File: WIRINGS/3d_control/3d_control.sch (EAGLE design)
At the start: 8 parts

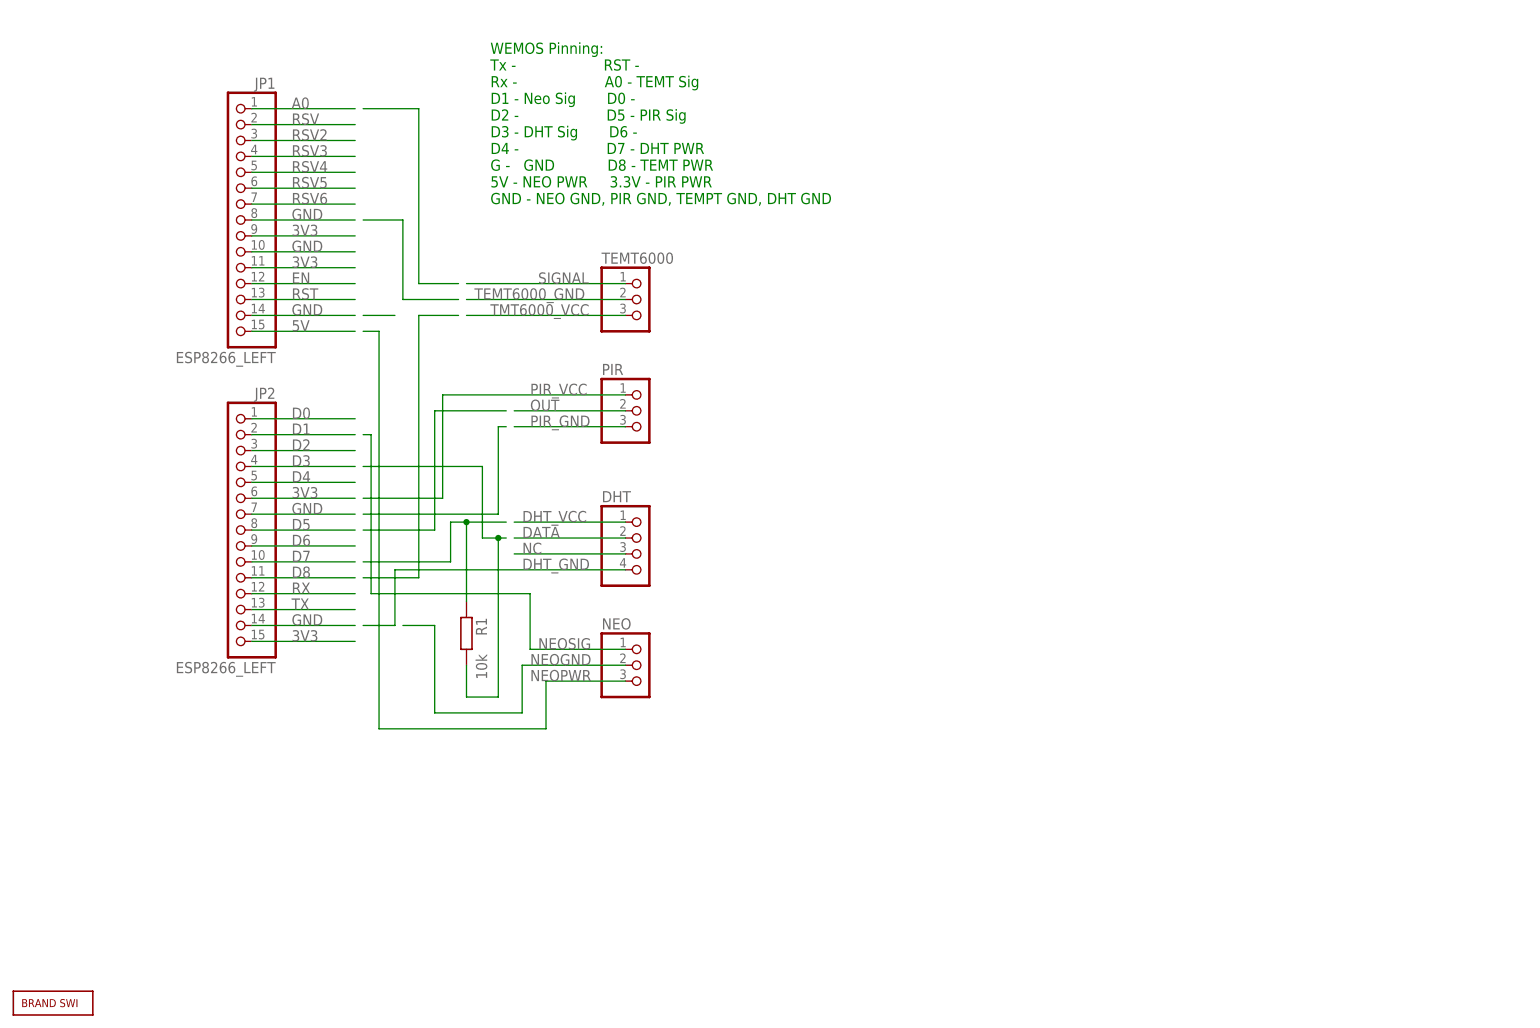
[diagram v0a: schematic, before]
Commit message: integration checkin
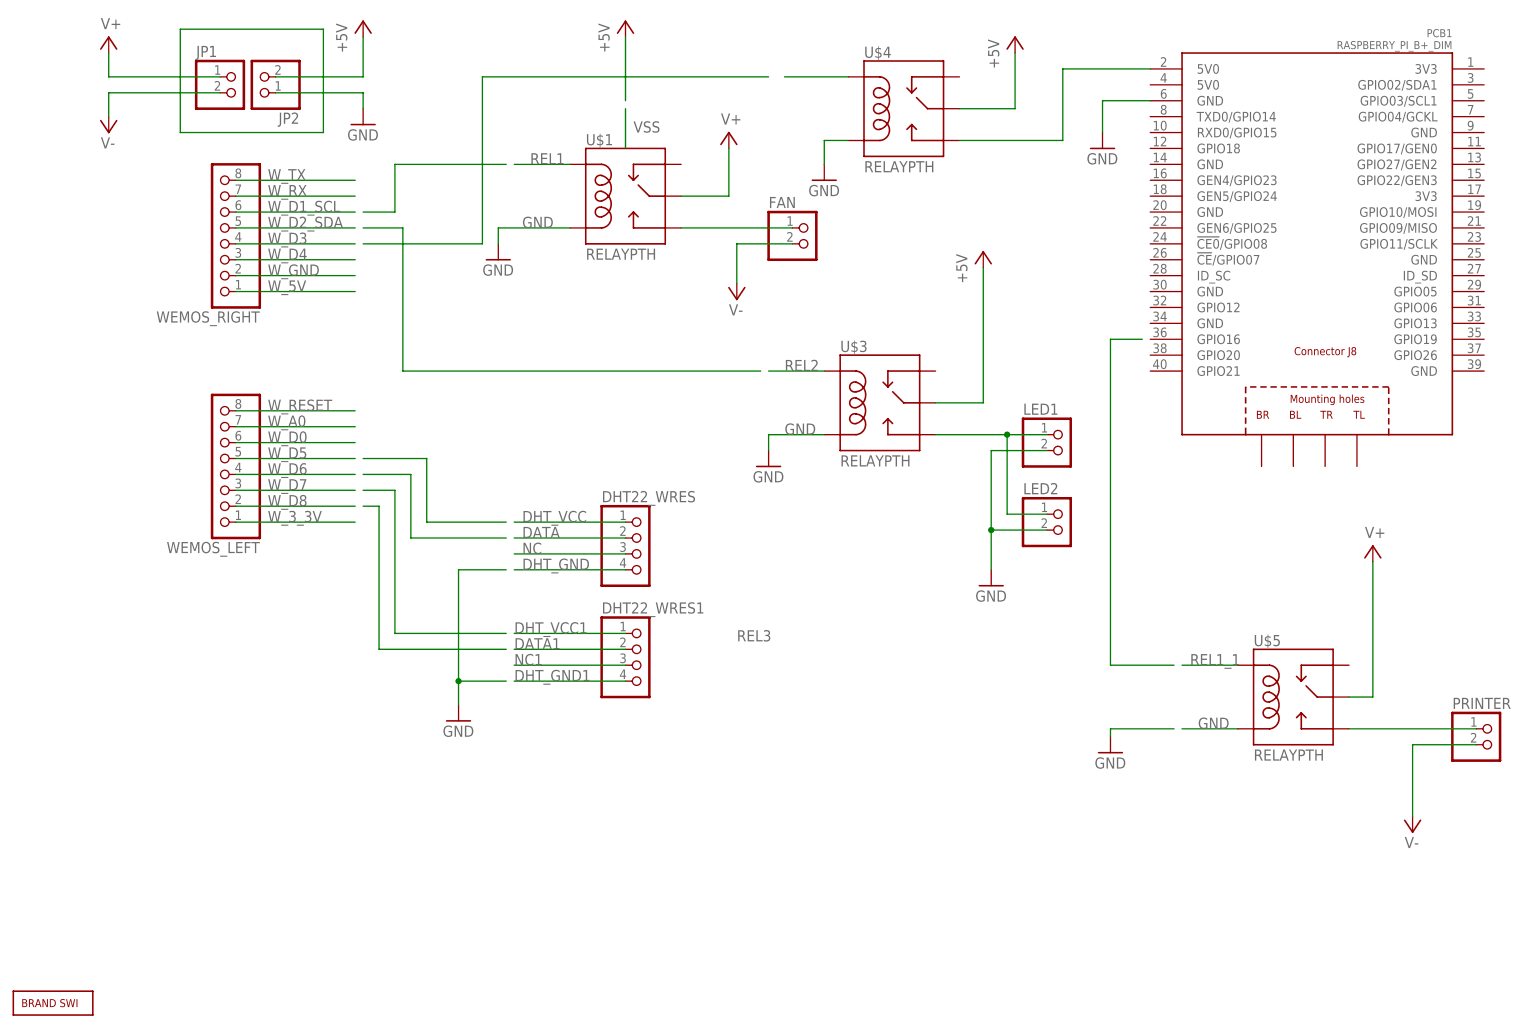
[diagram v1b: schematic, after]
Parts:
- removed NEO, PIR, TEMT6000: (no value), pinhead:PINHD-1X3
- removed R1: 10k, rcl:R-EU_0207/10
- added DHT22_WRES1: (no value), pinhead:PINHD-1X4
- added FAN, LED1, LED2, PRINTER: (no value), pinhead:PINHD-1X2
- added PCB1: RASPBERRY_PI_B+_DIM, SWI_COMMONS:RASPBERRY_PI_B+_DIM
- added U$1, U$3, U$4, U$5: RELAYPTH, SWI_COMMONS:RELAYPTH
- added WEMOS_LEFT, WEMOS_RIGHT: (no value), pinhead:PINHD-1X8
- JP1, JP2: value ESP8266_LEFT -> (none); device pinhead:PINHD-1X15 -> pinhead:PINHD-1X2
- renumbered DHT to DHT22_WRES
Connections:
- removed net 3V3: JP1.11, JP1.9, JP2.15, JP2.6
- removed net 5V: JP1.15
- removed net A0: JP1.1
- removed net D0: JP2.1
- removed net D1: JP2.2
- removed net D2: JP2.3
- removed net D3: JP2.4
- removed net D4: JP2.5
- removed net D5: JP2.8
- removed net D6: JP2.9
- removed net D7: JP2.10
- removed net D8: JP2.11
- removed net EN: JP1.12
- removed net N$3: R1.1
- removed net NEOGND: NEO.2
- removed net NEOPWR: NEO.3
- removed net NEOSIG: NEO.1
- removed net OUT: PIR.2
- removed net PIR_GND: PIR.3
- removed net PIR_VCC: PIR.1
- removed net RST: JP1.13
- removed net RSV: JP1.2
- removed net RSV2: JP1.3
- removed net RSV3: JP1.4
- removed net RSV4: JP1.5
- removed net RSV5: JP1.6
- removed net RSV6: JP1.7
- removed net RX: JP2.12
- removed net SIGNAL: TEMT6000.1
- removed net TEMT6000_GND: TEMT6000.2
- removed net TMT6000_VCC: TEMT6000.3
- removed net TX: JP2.13
- new net +5V: JP2.2, U$3.SWCOMMON, U$4.SWCOMMON
- new net DATA1: DHT22_WRES1.2
- new net DHT_GND1: DHT22_WRES1.4
- new net DHT_VCC1: DHT22_WRES1.1
- new net N$10: PCB1.5V0@1, U$4.SWOPEN
- new net N$13: PRINTER.1, U$5.SWOPEN
- new net N$9: FAN.1, U$1.SWOPEN
- new net NC1: DHT22_WRES1.3
- new net REL1: U$1.COIL1
- new net REL1_1: U$5.COIL1
- new net REL2: U$3.COIL1
- new net REL3: U$4.COIL1
- new net V+: JP1.1, U$1.SWCOMMON, U$5.SWCOMMON
- new net V-: FAN.2, JP1.2, PRINTER.2
- new net W_3_3V: WEMOS_LEFT.1
- new net W_5V: WEMOS_RIGHT.1
- new net W_A0: WEMOS_LEFT.7
- new net W_D0: WEMOS_LEFT.6
- new net W_D1_SCL: WEMOS_RIGHT.6
- new net W_D2_SDA: WEMOS_RIGHT.5
- new net W_D3: WEMOS_RIGHT.4
- new net W_D4: WEMOS_RIGHT.3
- new net W_D5: WEMOS_LEFT.5
- new net W_D6: WEMOS_LEFT.4
- new net W_D7: WEMOS_LEFT.3
- new net W_D8: WEMOS_LEFT.2
- new net W_GND: WEMOS_RIGHT.2
- new net W_RESET: WEMOS_LEFT.8
- new net W_RX: WEMOS_RIGHT.7
- new net W_TX: WEMOS_RIGHT.8
- net GND: now also JP2.1, LED1.2, LED2.2, PCB1.GND@8, U$1.COIL0, U$3.COIL0, U$4.COIL0, U$5.COIL0; no longer JP1.10, JP1.14, JP1.8, JP2.14, JP2.7
- net N$1: now also LED1.1, LED2.1; no longer R1.2
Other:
- note removed: "WEMOS Pinning: Tx - RST - Rx - A0 - TEMT Sig D1 - Neo Sig D0 - D2 - D5 - PIR Sig D3 - DHT Sig D6 - D4 - D7 - DHT PWR G - GND D8 - TEMT PWR 5V - NEO PWR 3.3V - PIR PWR GND - NEO GND, PIR GND, TEMPT GND, DHT GND"
